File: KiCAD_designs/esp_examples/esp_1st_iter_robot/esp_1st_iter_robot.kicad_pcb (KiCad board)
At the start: 2 copper layers, 63 x 45 mm, 23 parts, among them J1 B2B-PH-SM4-TBLFSN, J2 B2B-PH-SM4-TBLFSN, J3 Conn_01x02_Pin, J5 Conn_01x03_Pin, Q1 AO3400A, SW2 RS-282G05A3-SM RT, SW3 RS-282G05A3-SM RT, U1 ESP-12F, U2 AMS1117-3.3, U3 CPT-9019S-SMT-TR

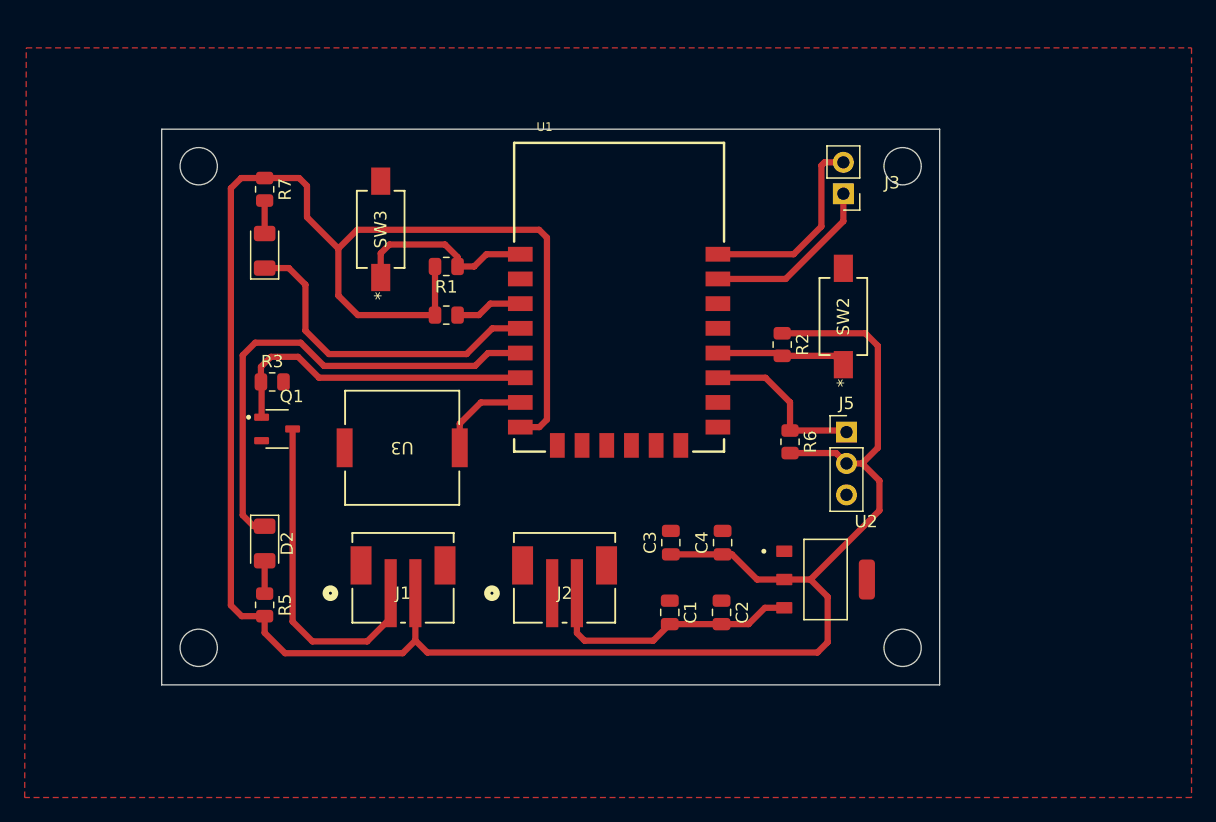
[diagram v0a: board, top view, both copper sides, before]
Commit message: esp_camRoller
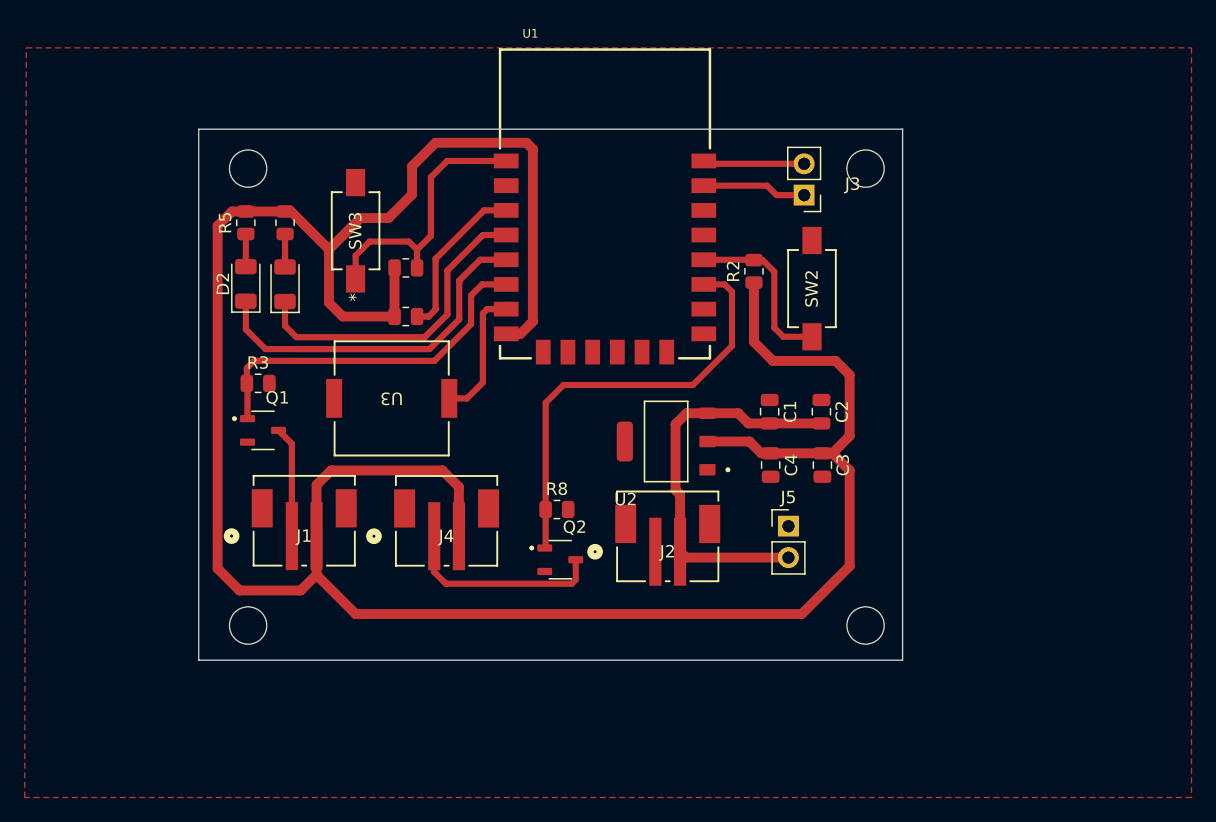
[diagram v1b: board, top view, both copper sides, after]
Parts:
- removed R6: R, Resistor_SMD:R_0805_2012Metric
- added J4: B2B-PH-SM4-TBLFSN, esp_lib:CONN_B2B-PH-SM4-TBLFSN_JST, F.Cu at (60.1, 56.7)
- added Q2: AO3400A, esp_lib:SOT95P280X125-3N, F.Cu at (69.3, 59.9)
- added R8: R, Resistor_SMD:R_0805_2012Metric, F.Cu at (69.0, 55.8)
- J5: value Conn_01x03_Pin -> Conn_01x02_Pin; footprint Connector_PinHeader_2.54mm:PinHeader_1x03_P2.54mm_Vertical -> Connector_PinHeader_2.54mm:PinHeader_1x02_P2.54mm_Vertical
- moved R5 31.0 mm to (43.8, 32.6), turned to 90 degrees
- moved D2 21.1 mm to (43.8, 37.5), turned to 90 degrees
- moved C1 18.2 mm to (86.2, 47.9)
- moved C2 18.2 mm to (90.4, 47.9)
- moved U2 17.1 mm to (77.9, 50.3), turned to 180 degrees
- moved C3 13.8 mm to (90.5, 52.2), turned to -90 degrees
- moved J1 9.24 mm to (48.5, 56.7)
- moved J2 9.00 mm to (78.0, 58.0)
- moved J5 8.95 mm to (87.8, 57.1)
- moved U1 7.64 mm to (72.9, 31.1)
- moved C4 7.39 mm to (86.3, 52.2), turned to -90 degrees
- moved R2 6.35 mm to (85.0, 36.5), turned to 90 degrees
- moved U3 4.09 mm to (55.6, 46.8)
- moved SW2 3.40 mm to (89.7, 37.9)
- moved R1 3.28 mm to (56.8, 36.2)
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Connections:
- C1 pad 2: Net-(U2-VIN) -> Net-(J5-Pin_2)
- C2 pad 2: Net-(U2-VIN) -> Net-(J5-Pin_2)
- J2 pad 2: Net-(U2-VIN) -> Net-(J5-Pin_2)
- J5 pad 1: /servo -> GND
- J5 pad 2: VCC -> Net-(J5-Pin_2)
- U1 pad 17: /servo -> /DC2
- U2 pad 3: Net-(U2-VIN) -> Net-(J5-Pin_2)
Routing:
- net /DC2: track 0.00 -> 35.7 mm
- net Net-(J5-Pin_2): track 0.00 -> 32.0 mm
- net Net-(U2-VIN): track 21.4 -> 0.00 mm
- net Net-(J4-Pad1): track 0.00 -> 16.5 mm
- net Net-(J1-Pad1): track 27.0 -> 10.5 mm
- net /servo: track 13.6 -> 0.00 mm
- net /LED1: track 39.2 -> 28.9 mm
- net Net-(J3-Pin_2): track 16.1 -> 8.22 mm
- net Net-(U1-EN): track 5.48 -> 13.2 mm
- net Net-(U1-RST): track 15.2 -> 22.1 mm
- net Net-(J3-Pin_1): track 14.3 -> 8.45 mm
- net /boot: track 10.6 -> 14.0 mm
- net /buzzer: track 7.57 -> 10.9 mm
- net /DC: track 26.1 -> 29.3 mm
- net VCC: track 208.1 -> 210.9 mm
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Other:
- board size 63 x 45 mm -> 57 x 43 mm
